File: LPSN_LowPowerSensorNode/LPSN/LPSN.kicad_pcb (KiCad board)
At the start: 2 copper layers, 33.3 x 29.2 mm, 9 parts, among them U2 SHT4x, U3 LPS22HB, U5 STM32U031F6Px

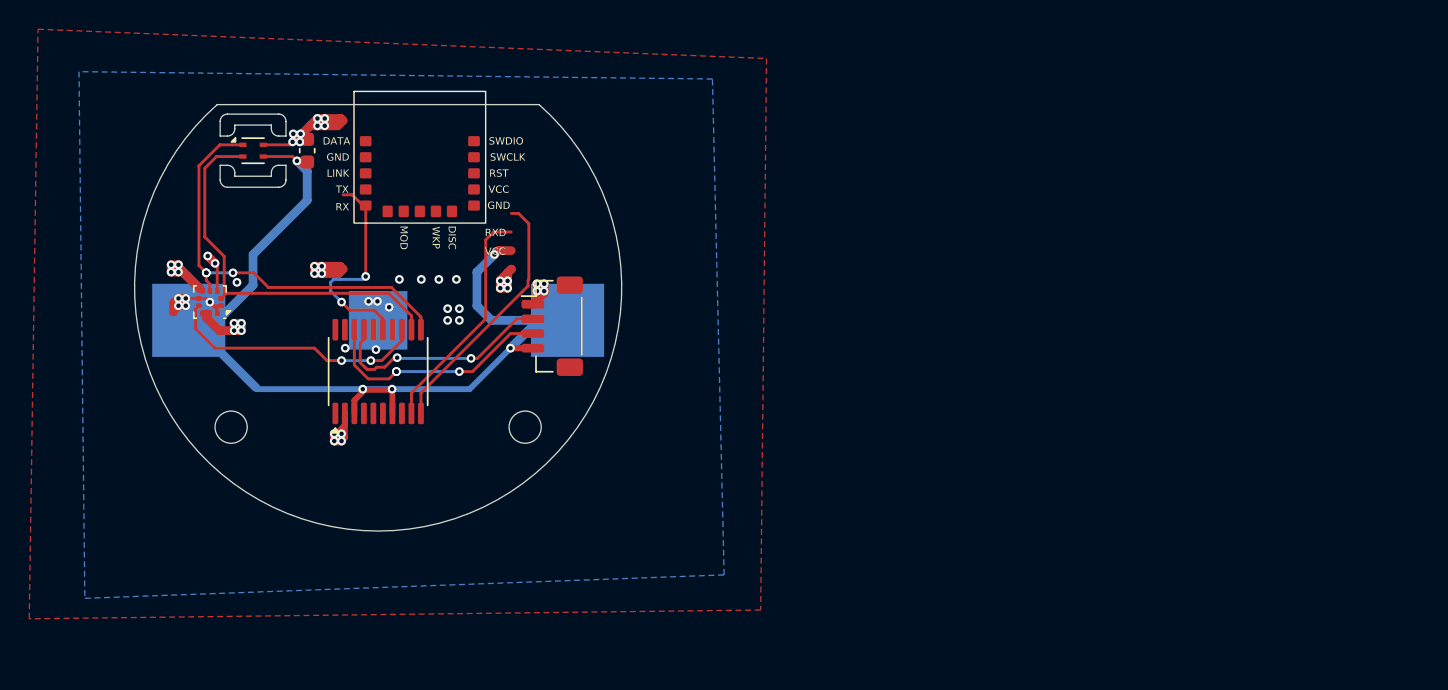
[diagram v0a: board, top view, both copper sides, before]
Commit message: LPSN - backup
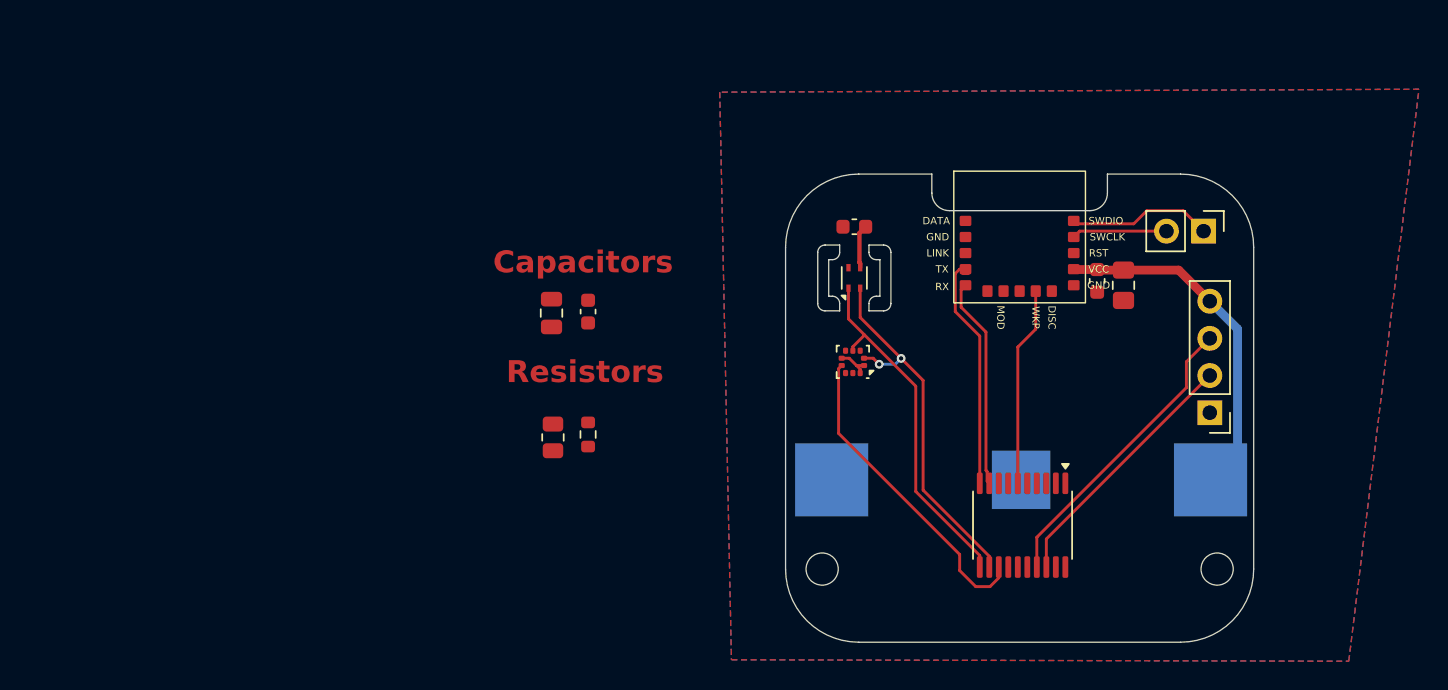
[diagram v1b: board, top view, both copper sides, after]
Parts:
- removed the ? at (153.8, 109.8)
- removed the ? at (133.7, 109.8)
- removed C3: 100n, Capacitor_SMD:C_0603_1608Metric
- removed STM_DB: JST_SH_BM04B-SRSS-TB_1x04-1MP_P1.00mm_Vertical, Connector_JST:JST_SH_BM04B-SRSS-TB_1x04-1MP_P1.00mm_Vertical
- added ?: , , F.Cu at (174.1, 119.5)
- added ?: , , F.Cu at (201.1, 119.5)
- added REF**: C_0603_1608Metric, Capacitor_SMD:C_0603_1608Metric, F.Cu at (192.9, 99.8)
- added REF**: R_0603_1608Metric, Resistor_SMD:R_0603_1608Metric, F.Cu at (158.1, 110.3)
- added REF**: C_0603_1608Metric, Capacitor_SMD:C_0603_1608Metric, F.Cu at (158.1, 101.9)
- added REF**: C_0805_2012Metric, Capacitor_SMD:C_0805_2012Metric, F.Cu at (155.6, 102.0)
- added REF**: C_0603_1608Metric, Capacitor_SMD:C_0603_1608Metric, F.Cu at (176.3, 96.1)
- added REF**: PinHeader_1x04_P2.54mm_Vertical, Connector_PinHeader_2.54mm:PinHeader_1x04_P2.54mm_Vertical, F.Cu at (200.6, 108.8)
- added REF**: PinHeader_1x02_P2.54mm_Vertical, Connector_PinHeader_2.54mm:PinHeader_1x02_P2.54mm_Vertical, F.Cu at (200.2, 96.4)
- added REF**: R_0805_2012Metric, Resistor_SMD:R_0805_2012Metric, F.Cu at (155.7, 110.5)
- added REF**: C_0805_2012Metric_Pad1.18x1.45mm_HandSolder, Capacitor_SMD:C_0805_2012Metric_Pad1.18x1.45mm_HandSolder, F.Cu at (194.7, 100.1)
- moved U5 45.3 mm to (187.8, 116.5), turned to -90 degrees
- moved BT1 45.3 mm to (187.7, 113.4), turned to 0 degrees
- moved U3 44.1 mm to (176.2, 105.3)
- moved U2 42.0 mm to (176.3, 99.6), turned to 90 degrees
- moved REF** 41.7 mm to (187.6, 96.8)
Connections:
- REF** pad 11: (no net) -> LPUART_TX
- REF** pad 12: (no net) -> LPUART_RX
- REF** pad 14: (no net) -> GND
- REF** pad 4: (no net) -> VCC
- REF** pad 5: (no net) -> GND
- REF** pad 7: (no net) -> GPIO_WAKEUP
- U5 pad 6: unconnected-(U5-PF2-Pad6) -> GPIO_WAKEUP
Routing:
- net VCC: track 76.2 -> 29.3 mm, vias 10 -> 0
- net GND: track 46.2 -> 0.00 mm, vias 48 -> 0
- net (no net): track 0.00 -> 16.9 mm
- net I2C_SDA: track 29.3 -> 24.2 mm, vias 3 -> 0
- net SW_CLK: track 15.8 -> 20.5 mm, vias 2 -> 0
- net PRESS_INT_READY: track 18.0 -> 21.6 mm, vias 2 -> 0
- net LPUART_TX: track 15.9 -> 14.5 mm
- net SW_DIO: track 16.3 -> 17.7 mm, vias 3 -> 0
- net I2C_SCL: track 26.9 -> 25.6 mm, vias 0 -> 2
- net LPUART_RX: track 17.5 -> 16.3 mm
- net GPIO_WAKEUP: track 14.9 -> 13.6 mm, vias 2 -> 0
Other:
- board size 33.3 x 29.2 mm -> 32 x 32 mm
- board text added: "Capacitors"
- board text added: "Resistors"
- board text removed: "RXD"
- board text removed: "VCC"
